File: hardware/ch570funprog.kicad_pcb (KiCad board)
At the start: 2 copper layers, 34.5 x 12.4 mm, 21 parts, among them J1 USB_C_Receptacle_USB2.0, J2 PGM, Q1 PMOS-SI2301CDS-T1-GE3, U1 USBLC6-2SC6, U2 AMS1117-3.3, U3 CH570Q, Y1 32M

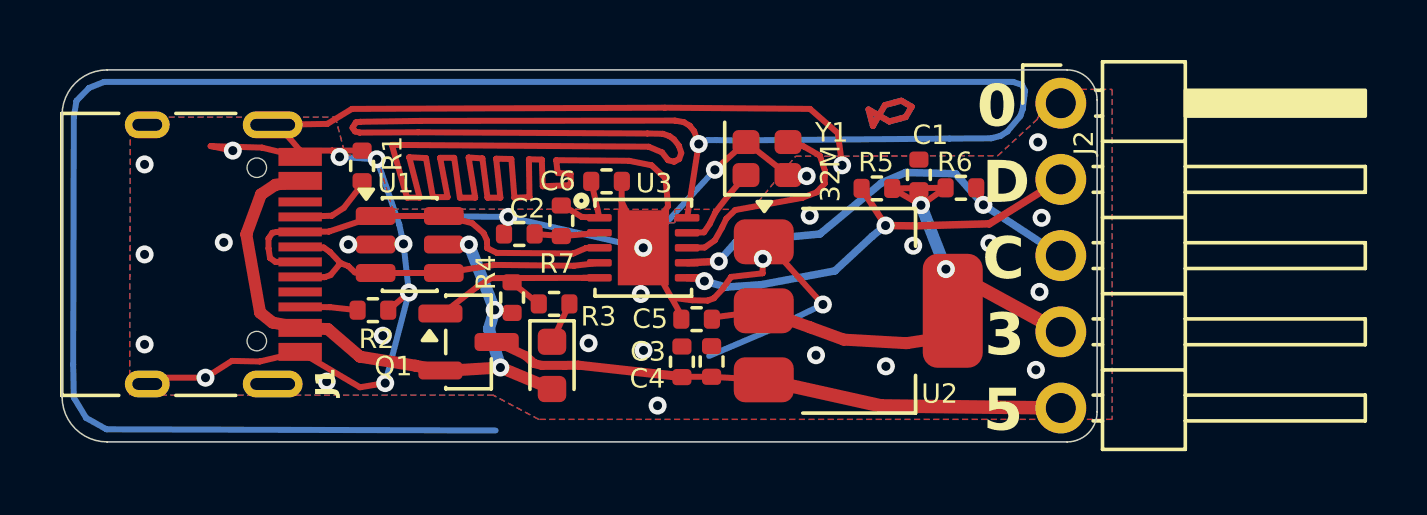
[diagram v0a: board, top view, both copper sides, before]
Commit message: Update to rev A
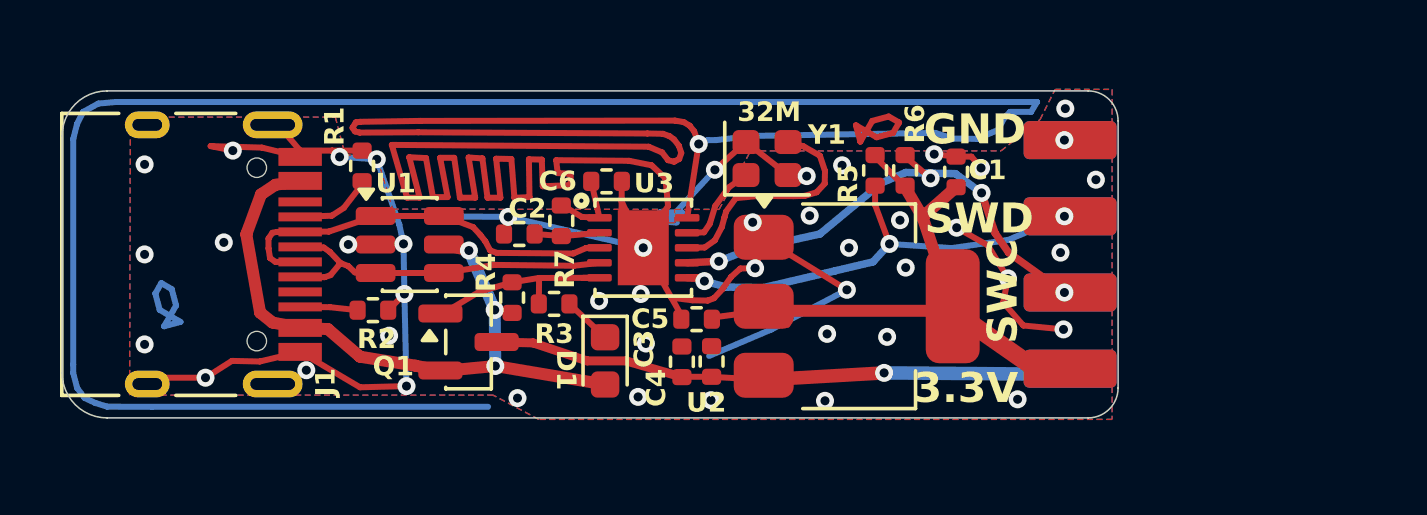
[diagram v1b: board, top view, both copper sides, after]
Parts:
- J2: footprint Connector_PinHeader_2.54mm:PinHeader_1x05_P2.54mm_Horizontal -> cnhardware:EDGE_02x04_2.54mm; moved to B.Cu
- moved J2 5.18 mm to (152.1, 82.2), turned to 90 degrees
- moved R6 1.95 mm to (148.1, 79.5), turned to 90 degrees
- moved D1 1.78 mm to (138.1, 85.8)
- moved C1 1.24 mm to (149.8, 79.5)
- moved R5 0.60 mm to (147.1, 79.5), turned to -90 degrees
- moved U2 0.15 mm to (146.5, 84.0)
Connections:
- J2 pad 1: GND -> PSWITCHED
- J2 pad 2: SWD -> VDD
- J2 pad 4: VDD -> SWC
- J2 pad 5: PSWITCHED -> SWD
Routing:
- net GND: track 213.1 -> 203.5 mm, vias 35 -> 46
- net SWC: track 15.0 -> 16.4 mm, vias 2 -> 4
- net +5V: track 21.6 -> 23.0 mm
- net VDD: track 22.3 -> 21.2 mm, vias 2 -> 0
- net PSWITCHED: track 19.1 -> 18.4 mm, vias 0 -> 1
- net SWD: track 15.0 -> 15.2 mm, vias 2 -> 3
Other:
- board size 34.5 x 12.4 mm -> 35.2 x 10.9 mm
- board text added: "1.6mm Thick Non-Lead HASL"
- board text added: "5.0V"
- board text added: "RX"
- board text added: "SCL"
- board text added: "SDA"
- board text added: "SWC"
- board text added: "SWD"
- board text added: "TX"
- board text removed: "0"
- board text removed: "1.0 or 0.8mm thick"
- board text removed: "3"
- board text removed: "5"
- board text removed: "5V"
- board text removed: "C"
- board text removed: "D"
- board text removed: "SWCLK"
- board text removed: "SWDIO"
